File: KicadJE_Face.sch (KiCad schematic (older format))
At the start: 70 parts, among them J101 Out1, J102 Out2, J103 In1.1, J104 In1.2, J105 In1.3, J106 In1.4, U101 TL072, U102 TL072

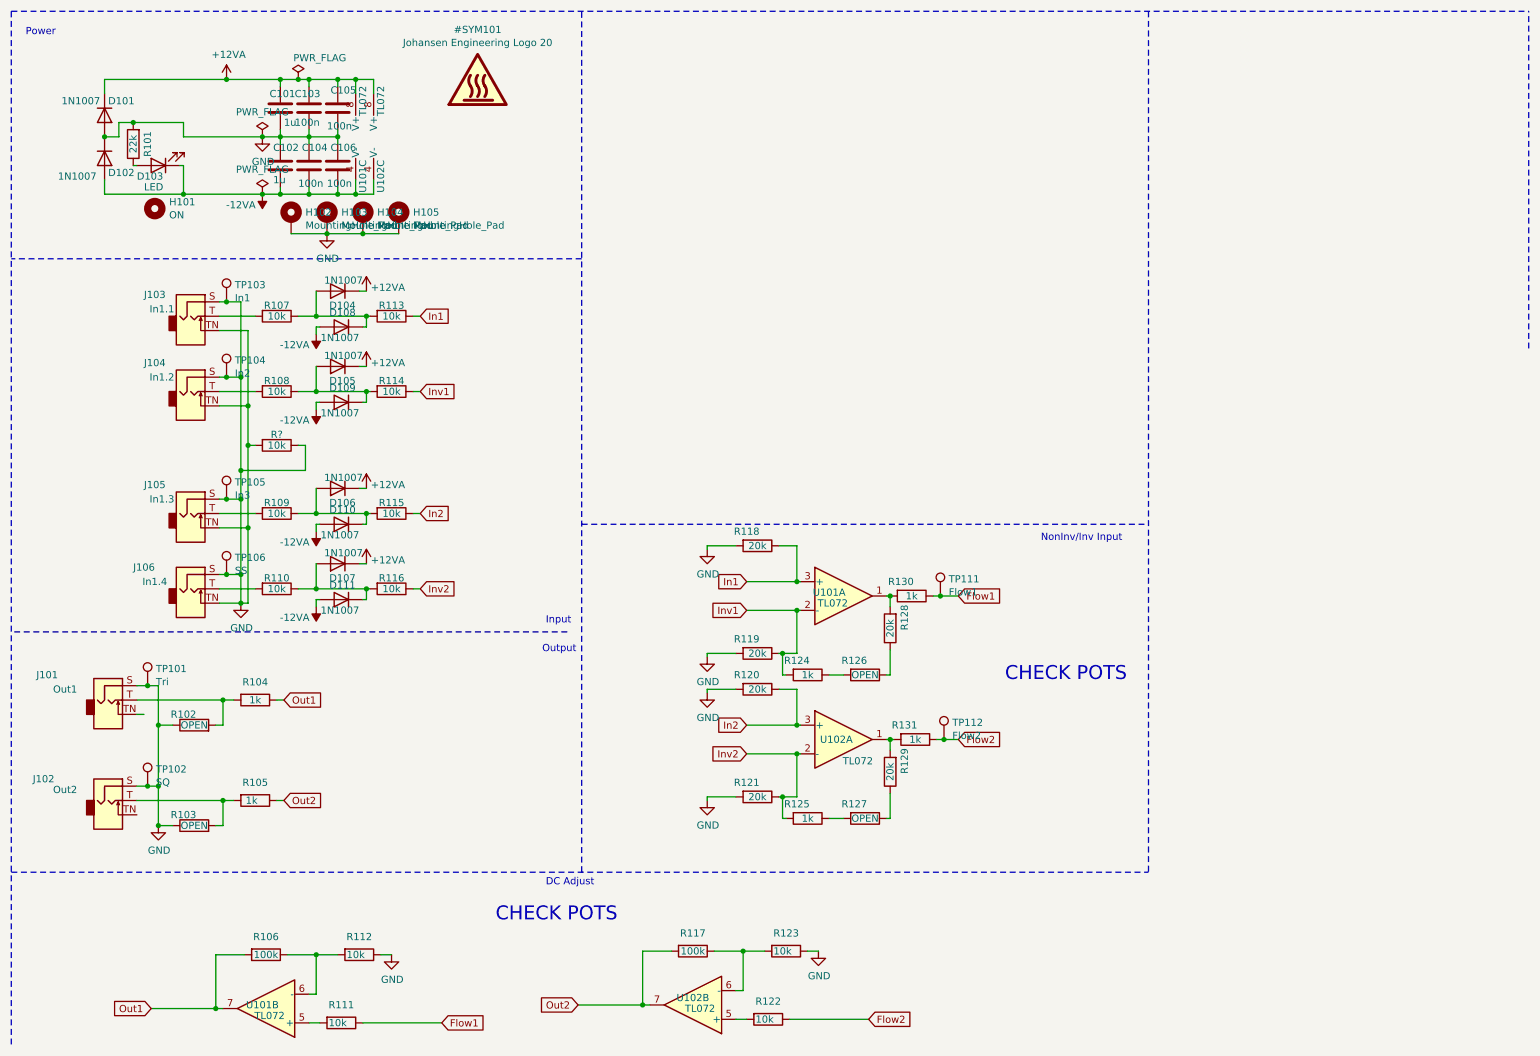
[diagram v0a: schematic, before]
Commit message: Schematic init
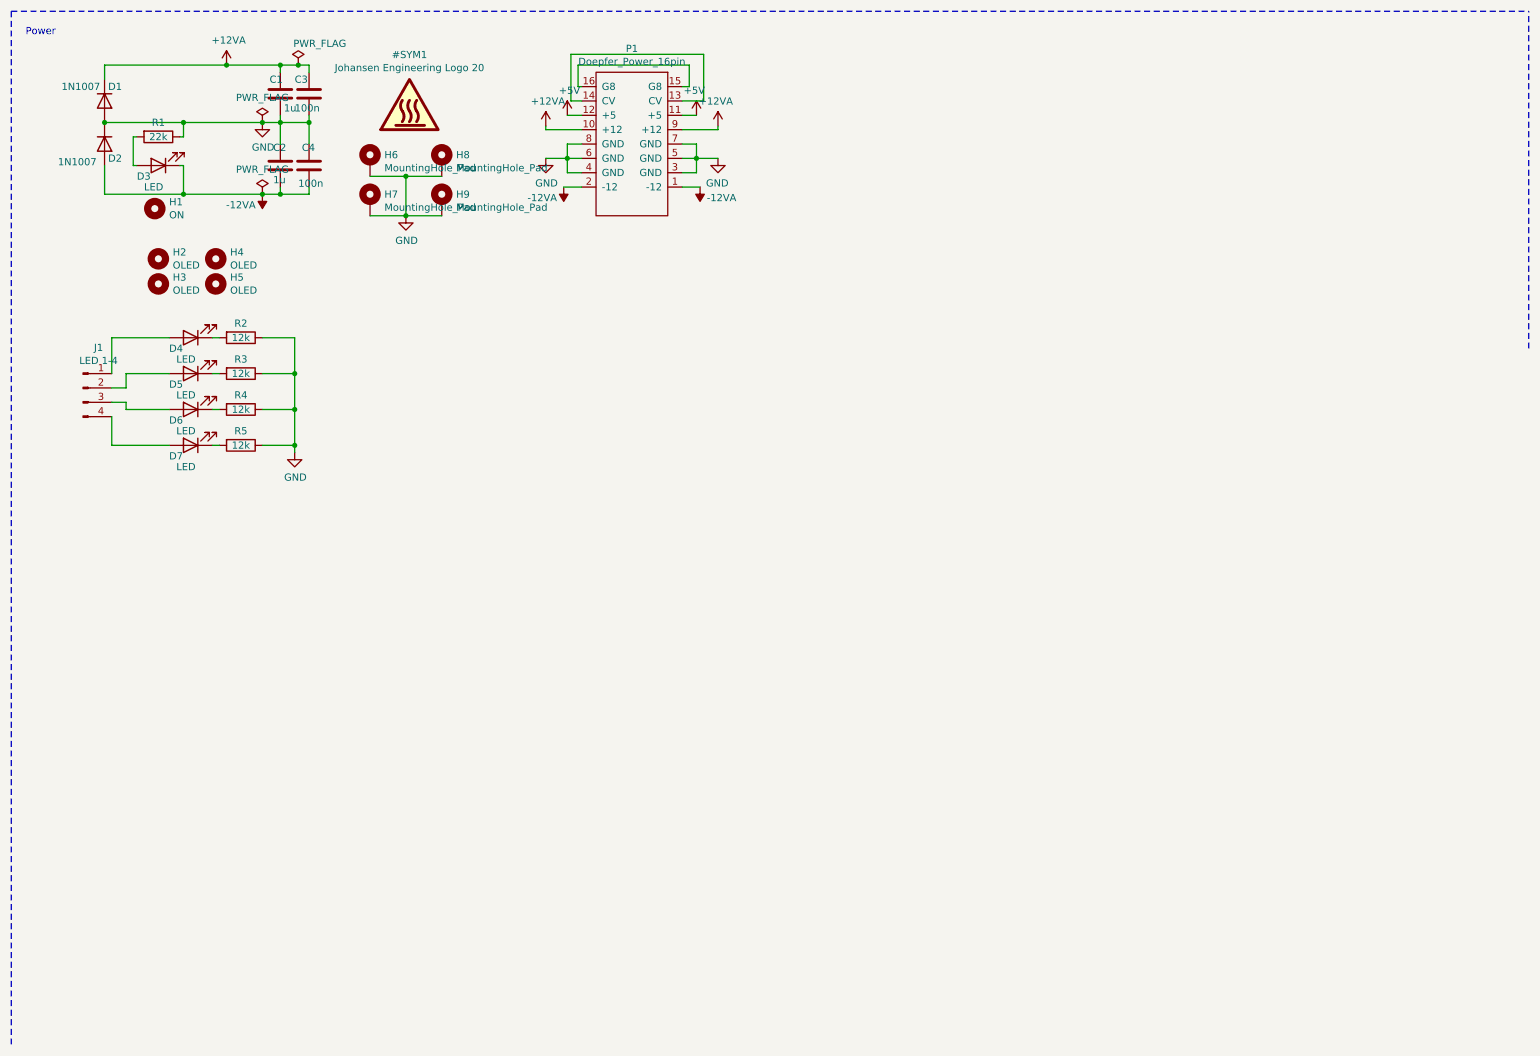
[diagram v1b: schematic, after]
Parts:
- removed C105, C106: 100n, Capacitor_SMD:C_0805_2012Metric_Pad1.15x1.40mm_HandSolder, symbol Device:C
- removed D104, D105, D106, D107, D108, D109, D110, D111: 1N1007, Diode_SMD:D_SOD-123, symbol Device:D
- removed J101: Out1, AJ-Dropbox-Kicad:PJ301SM, symbol Connector:AudioJack2_SwitchT
- removed J102: Out2, AJ-Dropbox-Kicad:PJ301SM, symbol Connector:AudioJack2_SwitchT
- removed J103: In1.1, AJ-Dropbox-Kicad:PJ301SM, symbol Connector:AudioJack2_SwitchT
- removed J104: In1.2, AJ-Dropbox-Kicad:PJ301SM, symbol Connector:AudioJack2_SwitchT
- removed J105: In1.3, AJ-Dropbox-Kicad:PJ301SM, symbol Connector:AudioJack2_SwitchT
- removed J106: In1.4, AJ-Dropbox-Kicad:PJ301SM, symbol Connector:AudioJack2_SwitchT
- removed R102, R103, R126, R127: OPEN, Resistor_SMD:R_0805_2012Metric_Pad1.15x1.40mm_HandSolder, symbol Device:R
- removed R104, R105, R124, R125, R130, R131: 1k, Resistor_SMD:R_0805_2012Metric_Pad1.15x1.40mm_HandSolder, symbol Device:R
- removed R106, R117: 100k, Resistor_SMD:R_0805_2012Metric_Pad1.15x1.40mm_HandSolder, symbol Device:R
- removed R107, R108, R109, R110, R111, R112, R113, R114, R115, R116, R122, R123, R?: 10k, Resistor_SMD:R_0805_2012Metric_Pad1.15x1.40mm_HandSolder, symbol Device:R
- removed R118, R119, R120, R121, R128, R129: 20k, Resistor_SMD:R_0805_2012Metric_Pad1.15x1.40mm_HandSolder, symbol Device:R
- removed TP101: Tri, AJ:Jack_6m3, symbol Connector:TestPoint
- removed TP102: SQ, AJ:Jack_6m3, symbol Connector:TestPoint
- removed TP103: In1, AJ:Jack_6m3, symbol Connector:TestPoint
- removed TP104: In2, AJ:Jack_6m3, symbol Connector:TestPoint
- removed TP105: In3, AJ:Jack_6m3, symbol Connector:TestPoint
- removed TP106: SS, AJ:Jack_6m3, symbol Connector:TestPoint
- removed TP111: Flow1, TestPoint:TestPoint_THTPad_2.0x2.0mm_Drill1.0mm, symbol Connector:TestPoint
- removed TP112: Flow2, TestPoint:TestPoint_THTPad_2.0x2.0mm_Drill1.0mm, symbol Connector:TestPoint
- removed U101, U102: TL072, AJ-Dropbox-Kicad:AJ_SO-8_5.3x6.2mm_P1.27mm, symbol Amplifier_Operational:TL072
- added D4, D5, D6, D7: LED, LED_SMD:LED_0805_2012Metric_Pad1.15x1.40mm_HandSolder, symbol Device:LED
- added H2, H3, H4, H5: OLED, MountingHole:MountingHole_2.7mm_M2.5, symbol Mechanical:MountingHole
- added J1: LED 1-4, Connector_PinSocket_2.54mm:PinSocket_1x04_P2.54mm_Vertical_SMD_Pin1Right, symbol Connector:Conn_01x04_Male
- added P1: Doepfer_Power_16pin, Connector_PinSocket_2.54mm:PinSocket_2x08_P2.54mm_Vertical_SMD, symbol Eurorack:Doepfer_Power_16pin
- added R2, R3, R4, R5: 12k, Resistor_SMD:R_0805_2012Metric_Pad1.15x1.40mm_HandSolder, symbol Device:R
- renumbered C101 to C1, C102 to C2, C103 to C3, C104 to C4, D101 to D1, D102 to D2, D103 to D3, H101 to H1, H103 to H6, H102 to H7, H105 to H8, H104 to H9, R101 to R1
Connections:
- net +12VA: now also P1.10 (+12), P1.9 (+12)
- net -12VA: now also P1.1 (-12), P1.2 (-12)
- net GND: now also R1.1, P1.3 (GND), P1.4 (GND), P1.5 (GND), P1.6 (GND), P1.7 (GND), P1.8 (GND), R2.1, R3.1, R4.1, R5.1; no longer R1.2
- net at D3.2 (A): now also R1.2; no longer R1.1
- new net: P1.13 (CV), P1.14 (CV)
- new net: P1.15 (G8), P1.16 (G8)
- new net: D4.1 (K), R2.2
- new net: D4.2 (A), J1.1 (Pin_1)
- new net: D5.1 (K), R3.2
- new net: D5.2 (A), J1.2 (Pin_2)
- new net: D6.1 (K), R4.2
- new net: D6.2 (A), J1.3 (Pin_3)
- new net: D7.1 (K), R5.2
- new net: D7.2 (A), J1.4 (Pin_4)
- new net +5V: P1.11 (+5), P1.12 (+5)
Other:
- note removed: "CHECK POTS"
- note removed: "DC Adjust"
- note removed: "Input"
- note removed: "NonInv/Inv Input"
- note removed: "Output"
- moved on the sheet: C1, C3, D1, D2, H6, H7, H8, H9, R1

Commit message: 6LED
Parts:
- added D8, D9: LED, AJ:D_0805_AJ, symbol Device:LED
- added R6, R7: 12k, AJ:R_0805_AJ, symbol Device:R
- C1, C2: footprint Capacitor_SMD:C_1206_3216Metric_Pad1.42x1.75mm_HandSolder -> Capacitor_SMD:C_1206_3216Metric
- C3, C4: footprint Capacitor_SMD:C_0805_2012Metric_Pad1.15x1.40mm_HandSolder -> AJ:C_0805_AJ
- D3, D4, D5, D6, D7: footprint LED_SMD:LED_0805_2012Metric_Pad1.15x1.40mm_HandSolder -> AJ:D_0805_AJ
- J1: value LED 1-4 -> LED 1-6; footprint Connector_PinSocket_2.54mm:PinSocket_1x04_P2.54mm_Vertical_SMD_Pin1Right -> Connector_PinSocket_2.54mm:PinSocket_1x06_P2.54mm_Vertical_SMD_Pin1Right; symbol Connector:Conn_01x04_Male -> Connector:Conn_01x06_Male
- R1, R2, R3, R4, R5: footprint Resistor_SMD:R_0805_2012Metric_Pad1.15x1.40mm_HandSolder -> AJ:R_0805_AJ
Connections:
- net GND: now also R6.1, R7.1
- new net: D8.2 (A), J1.5 (Pin_5)
- new net: D9.2 (A), J1.6 (Pin_6)
- new net: D8.1 (K), R6.2
- new net: D9.1 (K), R7.2
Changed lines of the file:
@@
 F 0 "C1" H 2325 1200 50  0000 L CNN
 F 1 "1u" H 2425 1000 50  0000 L CNN
-F 2 "Capacitor_SMD:C_1206_3216Metric_Pad1.42x1.75mm_HandSolder" H 2438 950 50  0001 C CNN
+F 2 "Capacitor_SMD:C_1206_3216Metric" H 2438 950 50  0001 C CNN
 F 3 "~" H 2400 1100 50  0001 C CNN
 	1    2400 1100
@@
 F 0 "C2" H 2350 1725 50  0000 L CNN
 F 1 "1u" H 2350 1500 50  0000 L CNN
-F 2 "Capacitor_SMD:C_1206_3216Metric_Pad1.42x1.75mm_HandSolder" H 2438 1450 50  0001 C CNN
+F 2 "Capacitor_SMD:C_1206_3216Metric" H 2438 1450 50  0001 C CNN
 F 3 "~" H 2400 1600 50  0001 C CNN
 	1    2400 1600
@@
 F 0 "R1" V 1450 1400 50  0000 C CNN
 F 1 "22k" V 1550 1400 50  0000 C CNN
-F 2 "Resistor_SMD:R_0805_2012Metric_Pad1.15x1.40mm_HandSolder" V 1480 1400 50  0001 C CNN
+F 2 "AJ:R_0805_AJ" V 1480 1400 50  0001 C CNN
 F 3 "~" H 1550 1400 50  0001 C CNN
 	1    1550 1400
@@
 F 0 "C3" H 2500 1200 50  0000 L CNN
 F 1 "100n" H 2500 1000 50  0000 L CNN
-F 2 "Capacitor_SMD:C_0805_2012Metric_Pad1.15x1.40mm_HandSolder" H 2638 950 50  0001 C CNN
+F 2 "AJ:C_0805_AJ" H 2638 950 50  0001 C CNN
 F 3 "~" H 2600 1100 50  0001 C CNN
 	1    2600 1100
@@
 F 0 "C4" H 2550 1725 50  0000 L CNN
 F 1 "100n" H 2525 1475 50  0000 L CNN
-F 2 "Capacitor_SMD:C_0805_2012Metric_Pad1.15x1.40mm_HandSolder" H 2638 1450 50  0001 C CNN
+F 2 "AJ:C_0805_AJ" H 2638 1450 50  0001 C CNN
 F 3 "~" H 2600 1600 50  0001 C CNN
 	1    2600 1600
@@
 F 0 "D3" H 1700 1675 50  0000 R CNN
 F 1 "LED" H 1650 1750 50  0000 R CNN
-F 2 "LED_SMD:LED_0805_2012Metric_Pad1.15x1.40mm_HandSolder" H 1550 1600 50  0001 C CNN
+F 2 "AJ:D_0805_AJ" H 1550 1600 50  0001 C CNN
 F 3 "~" H 1550 1600 50  0001 C CNN
 	1    1550 1600
@@
 F 0 "R2" V 2025 2800 50  0000 C CNN
 F 1 "12k" V 2125 2800 50  0000 C CNN
-F 2 "Resistor_SMD:R_0805_2012Metric_Pad1.15x1.40mm_HandSolder" V 2055 2800 50  0001 C CNN
+F 2 "AJ:R_0805_AJ" V 2055 2800 50  0001 C CNN
 F 3 "~" H 2125 2800 50  0001 C CNN
 	1    2125 2800
@@
 F 0 "D4" H 1925 2875 50  0000 R CNN
 F 1 "LED" H 1875 2950 50  0000 R CNN
-F 2 "LED_SMD:LED_0805_2012Metric_Pad1.15x1.40mm_HandSolder" H 1775 2800 50  0001 C CNN
+F 2 "AJ:D_0805_AJ" H 1775 2800 50  0001 C CNN
 F 3 "~" H 1775 2800 50  0001 C CNN
 	1    1775 2800
@@
 F 0 "R3" V 2025 3050 50  0000 C CNN
 F 1 "12k" V 2125 3050 50  0000 C CNN
-F 2 "Resistor_SMD:R_0805_2012Metric_Pad1.15x1.40mm_HandSolder" V 2055 3050 50  0001 C CNN
+F 2 "AJ:R_0805_AJ" V 2055 3050 50  0001 C CNN
 F 3 "~" H 2125 3050 50  0001 C CNN
 	1    2125 3050
@@
 F 0 "D5" H 1925 3125 50  0000 R CNN
 F 1 "LED" H 1875 3200 50  0000 R CNN
-F 2 "LED_SMD:LED_0805_2012Metric_Pad1.15x1.40mm_HandSolder" H 1775 3050 50  0001 C CNN
+F 2 "AJ:D_0805_AJ" H 1775 3050 50  0001 C CNN
 F 3 "~" H 1775 3050 50  0001 C CNN
 	1    1775 3050
@@
 F 0 "R4" V 2025 3300 50  0000 C CNN
 F 1 "12k" V 2125 3300 50  0000 C CNN
-F 2 "Resistor_SMD:R_0805_2012Metric_Pad1.15x1.40mm_HandSolder" V 2055 3300 50  0001 C CNN
+F 2 "AJ:R_0805_AJ" V 2055 3300 50  0001 C CNN
 F 3 "~" H 2125 3300 50  0001 C CNN
 	1    2125 3300
@@
 F 0 "D6" H 1925 3375 50  0000 R CNN
 F 1 "LED" H 1875 3450 50  0000 R CNN
-F 2 "LED_SMD:LED_0805_2012Metric_Pad1.15x1.40mm_HandSolder" H 1775 3300 50  0001 C CNN
+F 2 "AJ:D_0805_AJ" H 1775 3300 50  0001 C CNN
 F 3 "~" H 1775 3300 50  0001 C CNN
 	1    1775 3300
@@
 F 0 "R5" V 2025 3550 50  0000 C CNN
 F 1 "12k" V 2125 3550 50  0000 C CNN
-F 2 "Resistor_SMD:R_0805_2012Metric_Pad1.15x1.40mm_HandSolder" V 2055 3550 50  0001 C CNN
+F 2 "AJ:R_0805_AJ" V 2055 3550 50  0001 C CNN
 F 3 "~" H 2125 3550 50  0001 C CNN
 	1    2125 3550
@@
 F 0 "D7" H 1925 3625 50  0000 R CNN
 F 1 "LED" H 1875 3700 50  0000 R CNN
-F 2 "LED_SMD:LED_0805_2012Metric_Pad1.15x1.40mm_HandSolder" H 1775 3550 50  0001 C CNN
+F 2 "AJ:D_0805_AJ" H 1775 3550 50  0001 C CNN
 F 3 "~" H 1775 3550 50  0001 C CNN
 	1    1775 3550
@@
 	1925 3550 1975 3550
 $Comp
-L Connector:Conn_01x04_Male J1
+L Connector:Conn_01x06_Male J1
 U 1 1 6079C8D0
-P 1025 3150
-F 0 "J1" H 1133 3431 50  0000 C CNN
-F 1 "LED 1-4" H 1133 3340 50  0000 C CNN
-F 2 "Connector_PinSocket_2.54mm:PinSocket_1x04_P2.54mm_Vertical_SMD_Pin1Right" H 1025 3150 50  0001 C CNN
-F 3 "~" H 1025 3150 50  0001 C CNN
-	1    1025 3150
+P 1025 3250
+F 0 "J1" H 1133 3631 50  0000 C CNN
+F 1 "LED 1-6" H 1133 3540 50  0000 C CNN
+F 2 "Connector_PinSocket_2.54mm:PinSocket_1x06_P2.54mm_Vertical_SMD_Pin1Right" H 1025 3250 50  0001 C CNN
+F 3 "~" H 1025 3250 50  0001 C CNN
+	1    1025 3250
 	1    0    0    -1
 $EndComp
@@
 Wire Wire Line
 	1325 3300 1625 3300
-Wire Wire Line
-	1225 3350 1225 3550
-Wire Wire Line
-	1225 3550 1625 3550
 $Comp
 L power:GND #PWR04
 U 1 1 607A6BB6
-P 2500 3600
-F 0 "#PWR04" H 2500 3350 50  0001 C CNN
-F 1 "GND" H 2505 3427 50  0000 C CNN
-F 2 "" H 2500 3600 50  0001 C CNN
-F 3 "" H 2500 3600 50  0001 C CNN
-	1    2500 3600
-	1    0    0    -1
-$EndComp
-Wire Wire Line
-	2500 3600 2500 3550
+P 2500 4100
+F 0 "#PWR04" H 2500 3850 50  0001 C CNN
+F 1 "GND" H 2505 3927 50  0000 C CNN
+F 2 "" H 2500 4100 50  0001 C CNN
+F 3 "" H 2500 4100 50  0001 C CNN
+	1    2500 4100
+	1    0    0    -1
+$EndComp
 Wire Wire Line
 	2275 2800 2500 2800
@@
 	1    0    0    -1
 $EndComp
+$Comp
+L Device:R R6
+U 1 1 607D1243
+P 2125 3800
+AR Path="/607D1243" Ref="R6"  Part="1"
+AR Path="/5C8C5FC0/607D1243" Ref="R?"  Part="1"
+AR Path="/5CAAE8D3/607D1243" Ref="R?"  Part="1"
+AR Path="/5E4B0DD9/607D1243" Ref="R?"  Part="1"
+AR Path="/5E62ACA1/607D1243" Ref="R?"  Part="1"
+AR Path="/5F49A670/607D1243" Ref="R?"  Part="1"
+F 0 "R6" V 2025 3800 50  0000 C CNN
+F 1 "12k" V 2125 3800 50  0000 C CNN
+F 2 "AJ:R_0805_AJ" V 2055 3800 50  0001 C CNN
+F 3 "~" H 2125 3800 50  0001 C CNN
+	1    2125 3800
+	0    1    1    0
+$EndComp
+$Comp
+L Device:LED D?
+U 1 1 607D1541
+P 1775 3800
+AR Path="/5E4B0DD9/607D1541" Ref="D?"  Part="1"
+AR Path="/5E62ACA1/607D1541" Ref="D?"  Part="1"
+AR Path="/5F49A670/607D1541" Ref="D?"  Part="1"
+AR Path="/607D1541" Ref="D8"  Part="1"
+F 0 "D8" H 1925 3875 50  0000 R CNN
+F 1 "LED" H 1875 3950 50  0000 R CNN
+F 2 "AJ:D_0805_AJ" H 1775 3800 50  0001 C CNN
+F 3 "~" H 1775 3800 50  0001 C CNN
+	1    1775 3800
+	-1   0    0    1
+$EndComp
+Wire Wire Line
+	1925 3800 1975 3800
+$Comp
+L Device:R R7
+U 1 1 607D154C
+P 2125 4050
+AR Path="/607D154C" Ref="R7"  Part="1"
+AR Path="/5C8C5FC0/607D154C" Ref="R?"  Part="1"
+AR Path="/5CAAE8D3/607D154C" Ref="R?"  Part="1"
+AR Path="/5E4B0DD9/607D154C" Ref="R?"  Part="1"
+AR Path="/5E62ACA1/607D154C" Ref="R?"  Part="1"
+AR Path="/5F49A670/607D154C" Ref="R?"  Part="1"
+F 0 "R7" V 2025 4050 50  0000 C CNN
+F 1 "12k" V 2125 4050 50  0000 C CNN
+F 2 "AJ:R_0805_AJ" V 2055 4050 50  0001 C CNN
+F 3 "~" H 2125 4050 50  0001 C CNN
+	1    2125 4050
+	0    1    1    0
+$EndComp
+$Comp
+L Device:LED D?
+U 1 1 607D1556
+P 1775 4050
+AR Path="/5E4B0DD9/607D1556" Ref="D?"  Part="1"
+AR Path="/5E62ACA1/607D1556" Ref="D?"  Part="1"
+AR Path="/5F49A670/607D1556" Ref="D?"  Part="1"
+AR Path="/607D1556" Ref="D9"  Part="1"
+F 0 "D9" H 1925 4125 50  0000 R CNN
+F 1 "LED" H 1875 4200 50  0000 R CNN
+F 2 "AJ:D_0805_AJ" H 1775 4050 50  0001 C CNN
+F 3 "~" H 1775 4050 50  0001 C CNN
+	1    1775 4050
+	-1   0    0    1
+$EndComp
+Wire Wire Line
+	1925 4050 1975 4050
+Wire Wire Line
+	2275 3800 2500 3800
+Wire Wire Line
+	2275 4050 2500 4050
+Wire Wire Line
+	2500 3550 2500 3800
+Connection ~ 2500 3800
+Wire Wire Line
+	2500 3800 2500 4050
+Connection ~ 2500 4050
+Wire Wire Line
+	2500 4050 2500 4100
+Wire Wire Line
+	1625 3550 1500 3550
+Wire Wire Line
+	1500 3550 1500 3350
+Wire Wire Line
+	1500 3350 1225 3350
+Wire Wire Line
+	1225 3450 1375 3450
+Wire Wire Line
+	1375 3450 1375 3800
+Wire Wire Line
+	1375 3800 1625 3800
+Wire Wire Line
+	1625 4050 1250 4050
+Wire Wire Line
+	1250 4050 1250 3550
+Wire Wire Line
+	1250 3550 1225 3550
 $EndSCHEMATC
